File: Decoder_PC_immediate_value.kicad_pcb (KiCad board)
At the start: 4 copper layers, 66.4 x 51.2 mm, 13 parts

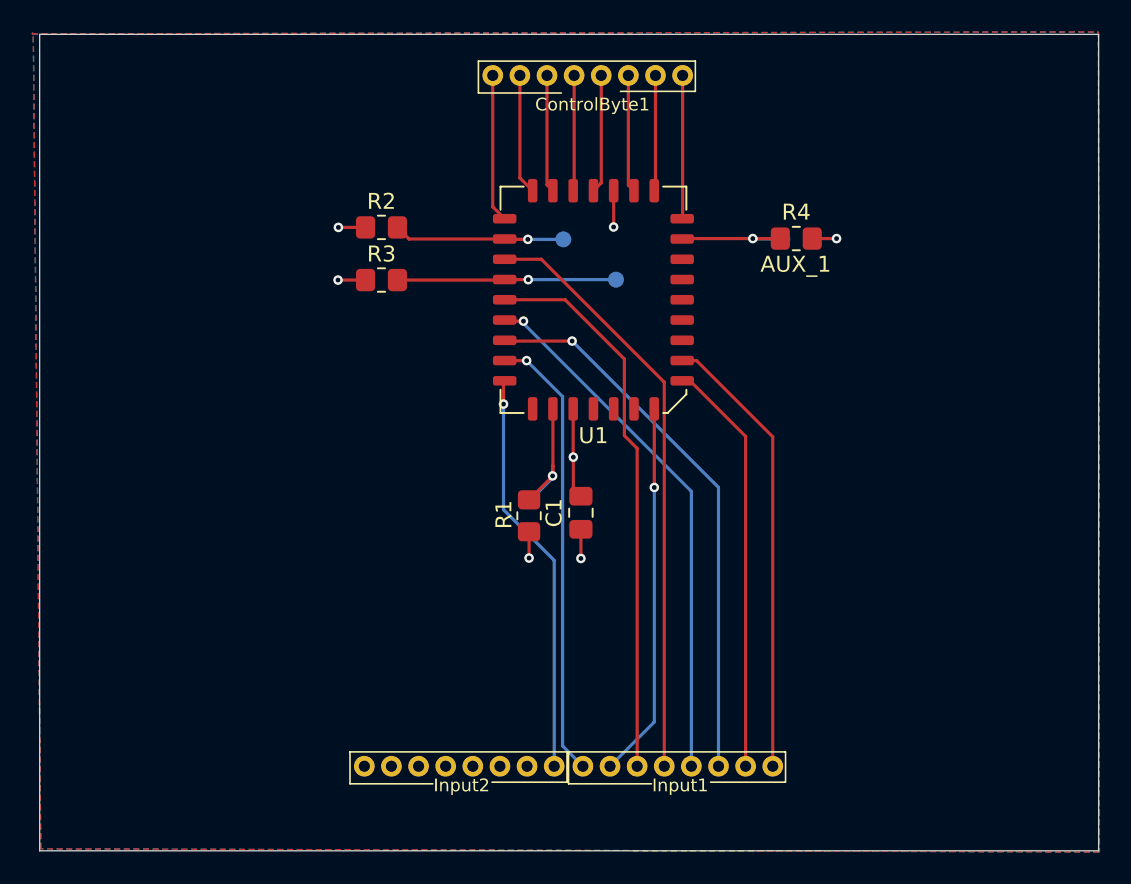
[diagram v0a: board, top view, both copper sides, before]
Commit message: Finished Decoder Design
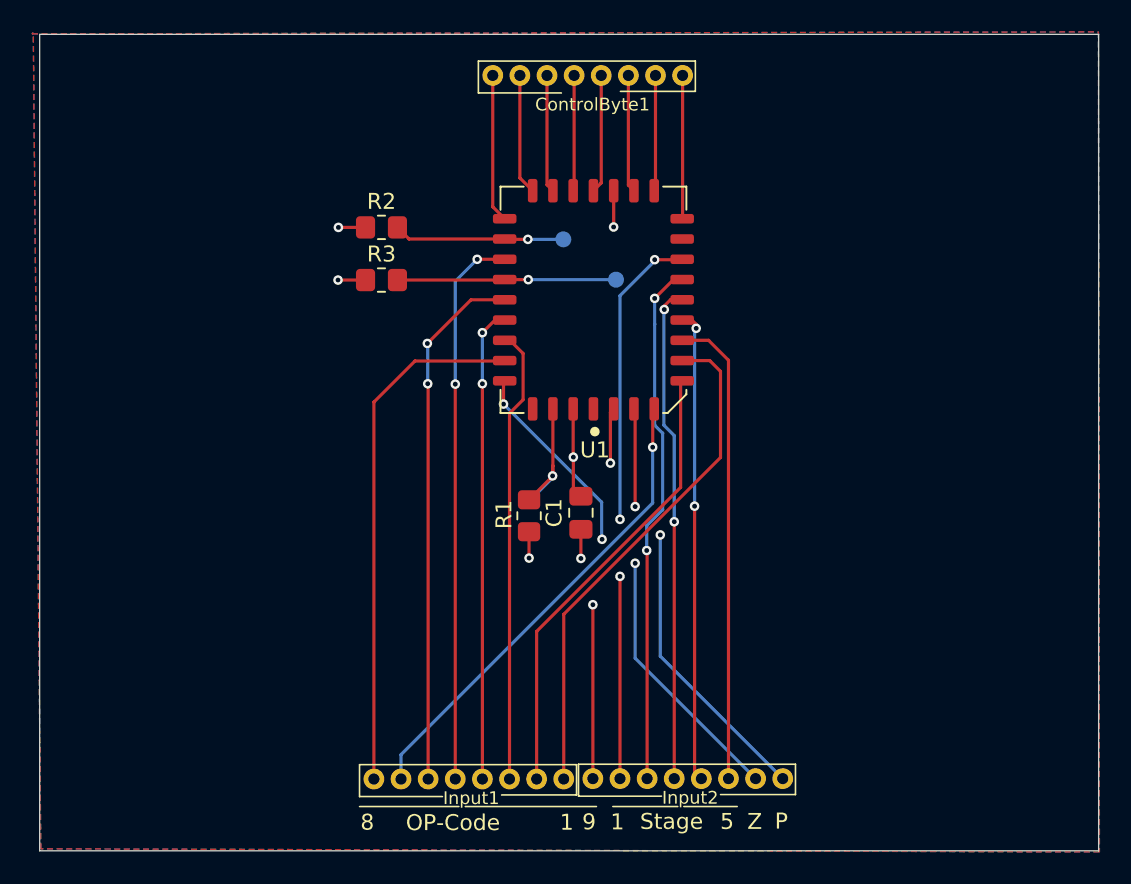
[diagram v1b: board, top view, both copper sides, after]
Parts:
- removed R4: 330Ω, Resistor_SMD:R_0805_2012Metric_Pad1.20x1.40mm_HandSolder
- removed TP4: AUX1, TestPoint:TestPoint_Pad_D1.0mm
- moved Input2 14.3 mm to (100.8, 105.2)
- moved Input1 13.1 mm to (87.0, 105.2)
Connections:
- Input2 pad 1: OP_Code_9 -> PM
- Input2 pad 2: unconnected-(Input2-Pad2) -> ZF
- Input2 pad 3: unconnected-(Input2-Pad3) -> Stage_5
- Input2 pad 4: unconnected-(Input2-Pad4) -> Stage_4
- Input2 pad 5: unconnected-(Input2-Pad5) -> Stage_3
- Input2 pad 6: unconnected-(Input2-Pad6) -> Stage_2
- Input2 pad 7: unconnected-(Input2-Pad7) -> Stage_1
- Input2 pad 8: unconnected-(Input2-Pad8) -> OP_Code_9
- U1 pad 12: AUX_1 -> /CLK
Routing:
- net Stage_1: track 0.00 -> 35.2 mm, vias 0 -> 3
- net Stage_2: track 0.00 -> 32.9 mm, vias 0 -> 2
- net Stage_3: track 0.00 -> 31.2 mm, vias 0 -> 2
- net Stage_4: track 0.00 -> 29.7 mm, vias 0 -> 2
- net Stage_5: track 0.00 -> 29.6 mm
- net PM: track 0.00 -> 27.7 mm, vias 0 -> 2
- net ZF: track 0.00 -> 26.3 mm, vias 0 -> 2
- net AUX_1: track 8.02 -> 0.00 mm, vias 1 -> 0
- net OP_Code_7: track 23.6 -> 29.8 mm
- net OP_Code_3: track 34.7 -> 28.6 mm, vias 1 -> 0
- net OP_Code_8: track 28.3 -> 32.9 mm, vias 1 -> 0
- net OP_Code_1: track 28.3 -> 32.3 mm
- net OP_Code_4: track 33.5 -> 29.8 mm, vias 1 -> 2
- net OP_Code_2: track 26.1 -> 29.2 mm
- net OP_Code_5: track 37.3 -> 34.9 mm, vias 0 -> 2
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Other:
- board text added: "1"
- board text added: "5"
- board text added: "8"
- board text added: "9"
- board text added: "OP-Code"
- board text added: "P"
- board text added: "Stage"
- board text added: "Z"
- board text removed: "AUX1"
- board text removed: "AUX_1"
